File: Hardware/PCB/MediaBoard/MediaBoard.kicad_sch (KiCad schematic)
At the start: 45 parts, among them J1 Conn_01x07, J2 Conn_01x07, J3 Micro_SD_Card_Det_Hirose_DM3AT, J4 Conn_01x07, J5 Conn_01x07, J6 RGBLED, U1 RaspberryPi-Pico, U2 MAX98357

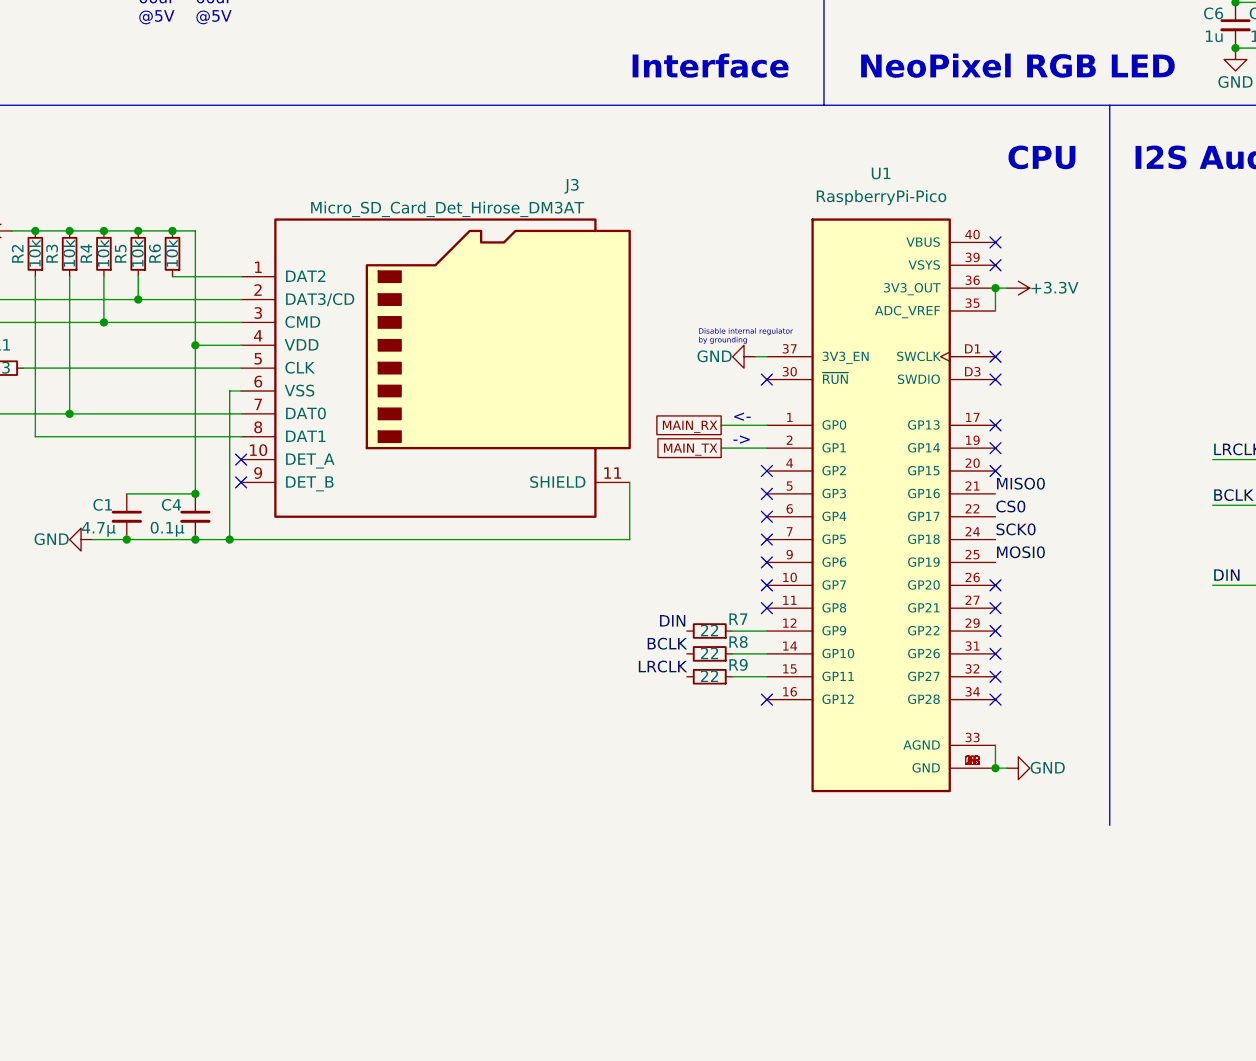
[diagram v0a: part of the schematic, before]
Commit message: もろもろ更新
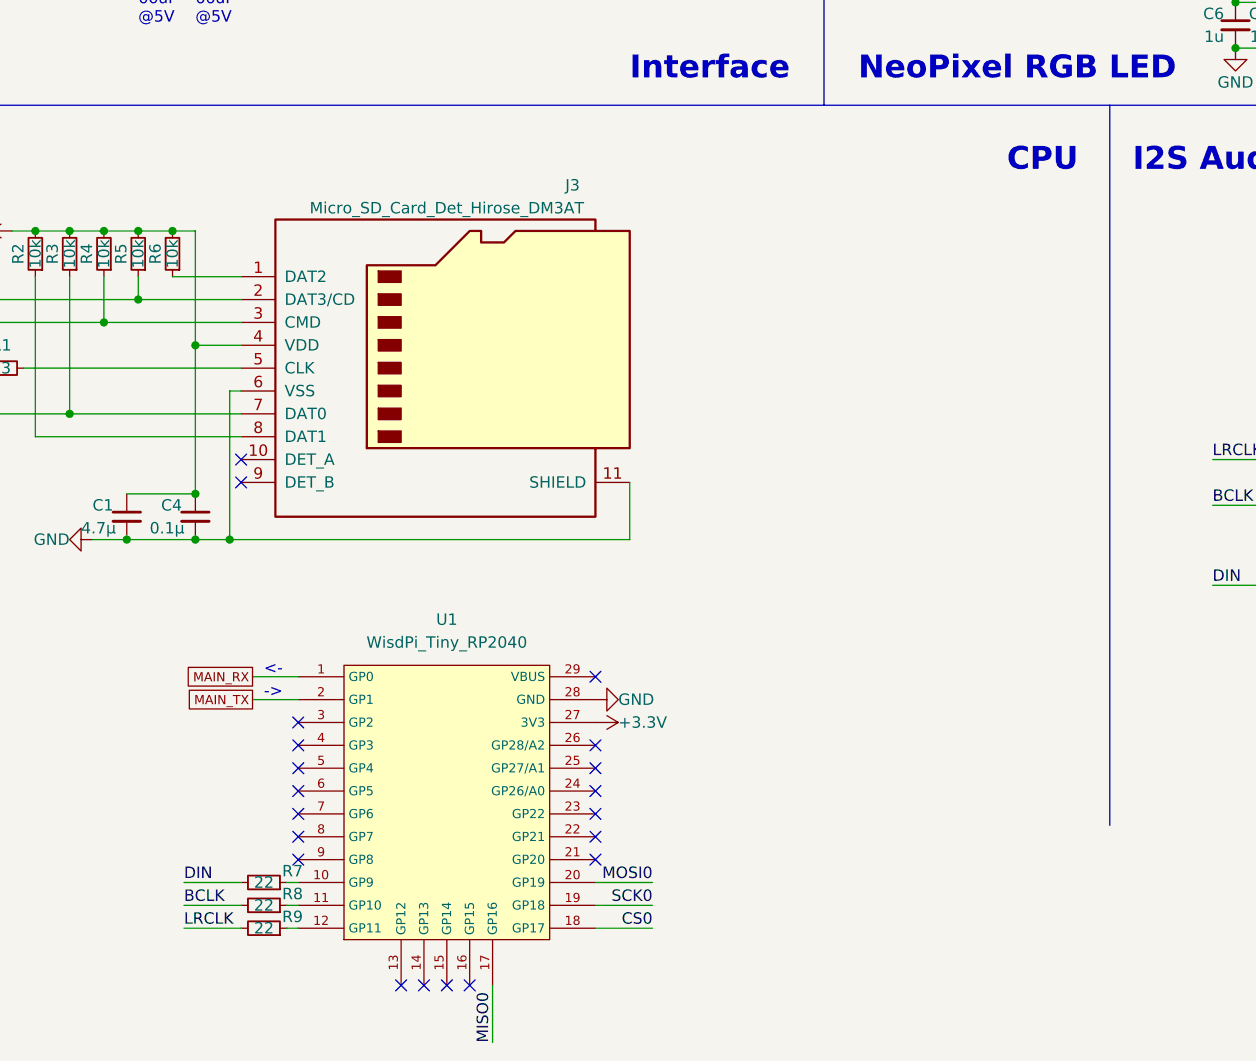
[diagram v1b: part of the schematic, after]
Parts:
- removed U1: RaspberryPi-Pico, Module_extlib:RaspberryPi-Pico, symbol MCU_Module_extlib:RaspberryPi-Pico
- added U1: WisdPi_Tiny_RP2040, Module_extlib:WisdPi_Tiny_RP2040, symbol MCU_Module_extlib:WisdPi_Tiny_RP2040
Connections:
- net +3.3V: now also U1.27 (3V3)
- net CS0: now also U1.18 (GP17)
- net GND: now also U1.28 (GND)
- net MAIN_RX: now also U1.1 (GP0)
- net MAIN_TX: now also U1.2 (GP1)
- net MISO0: now also U1.17 (GP16)
- net MOSI0: now also U1.20 (GP19)
- net SCK0: now also U1.19 (GP18)
- net at R9.1: now also U1.12 (GP11)
- net at R8.1: now also U1.11 (GP10)
- net at R7.1: now also U1.10 (GP9)
- no-connect marks 49 -> 45
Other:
- note removed: "Disable internal regulator by grounding"
- moved on the sheet: R7, R8, R9
